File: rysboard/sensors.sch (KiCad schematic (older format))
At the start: 11 parts, among them J10 ToF1, J11 ToF2, J12 ToF3, J13 ToF4, J15 ToF5, J16 ToF6, J9 IMU, Q10 DMP3036SSD-13, Q7 NST847BDP6T5G

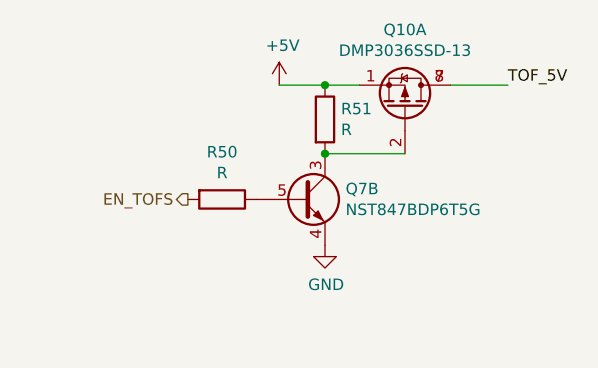
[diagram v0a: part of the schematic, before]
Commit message: Fixed library, added a few MOSFET layouts
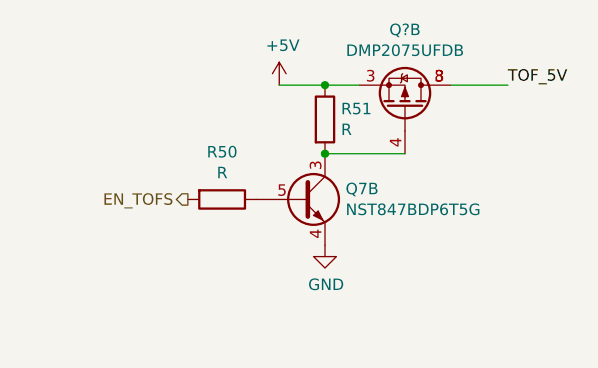
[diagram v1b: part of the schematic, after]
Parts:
- removed Q10: DMP3036SSD-13, Package_SO:SO-8_5.3x6.2mm_P1.27mm, symbol rysboard:DMP3036SSD-13
- added Q?: DMP2075UFDB, SamacSys_Parts:DMP2075UFDB7, symbol rysboard:DMP2075UFDB
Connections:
- net +5V: now also Q?.3 (S2)
- net TOF_5V: now also Q?.3 (S2), Q?.8 (D2_2)
- net at Q7.3 (C2), R51.2: now also Q?.4 (G2)
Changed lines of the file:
@@
 	2050 3700 2600 3700
-$Comp
-L rysboard:DMP3036SSD-13 Q10
-U 1 1 6035FE64
-P 5250 1350
-F 0 "Q10" V 5592 1350 50  0000 C CNN
-F 1 "DMP3036SSD-13" V 5501 1350 50  0000 C CNN
-F 2 "Package_SO:SO-8_5.3x6.2mm_P1.27mm" H 5450 1275 50  0001 L CIN
-F 3 "http://www.vishay.com/docs/70209/70209.pdf" H 5250 1350 50  0001 L CNN
-	1    5250 1350
-	0    1    -1   0
-$EndComp
 $Comp
 L power:+5V #PWR0102
@@
 Wire Wire Line
 	5700 1250 5450 1250
+$Comp
+L rysboard:DMP2075UFDB Q?
+U 2 1 605EBA08
+P 5250 1350
+F 0 "Q?" V 5592 1350 50  0000 C CNN
+F 1 "DMP2075UFDB" V 5501 1350 50  0000 C CNN
+F 2 "SamacSys_Parts:DMP2075UFDB7" H 5450 1275 50  0001 L CIN
+F 3 "" H 5250 1350 50  0001 L CNN
+	2    5250 1350
+	0    1    -1   0
+$EndComp
 $EndSCHEMATC
